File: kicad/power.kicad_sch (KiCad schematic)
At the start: 44 parts, among them J12 PJ-002B, U23 AP62300Z6, U24 AP62300Z6, U25 AP62300Z6

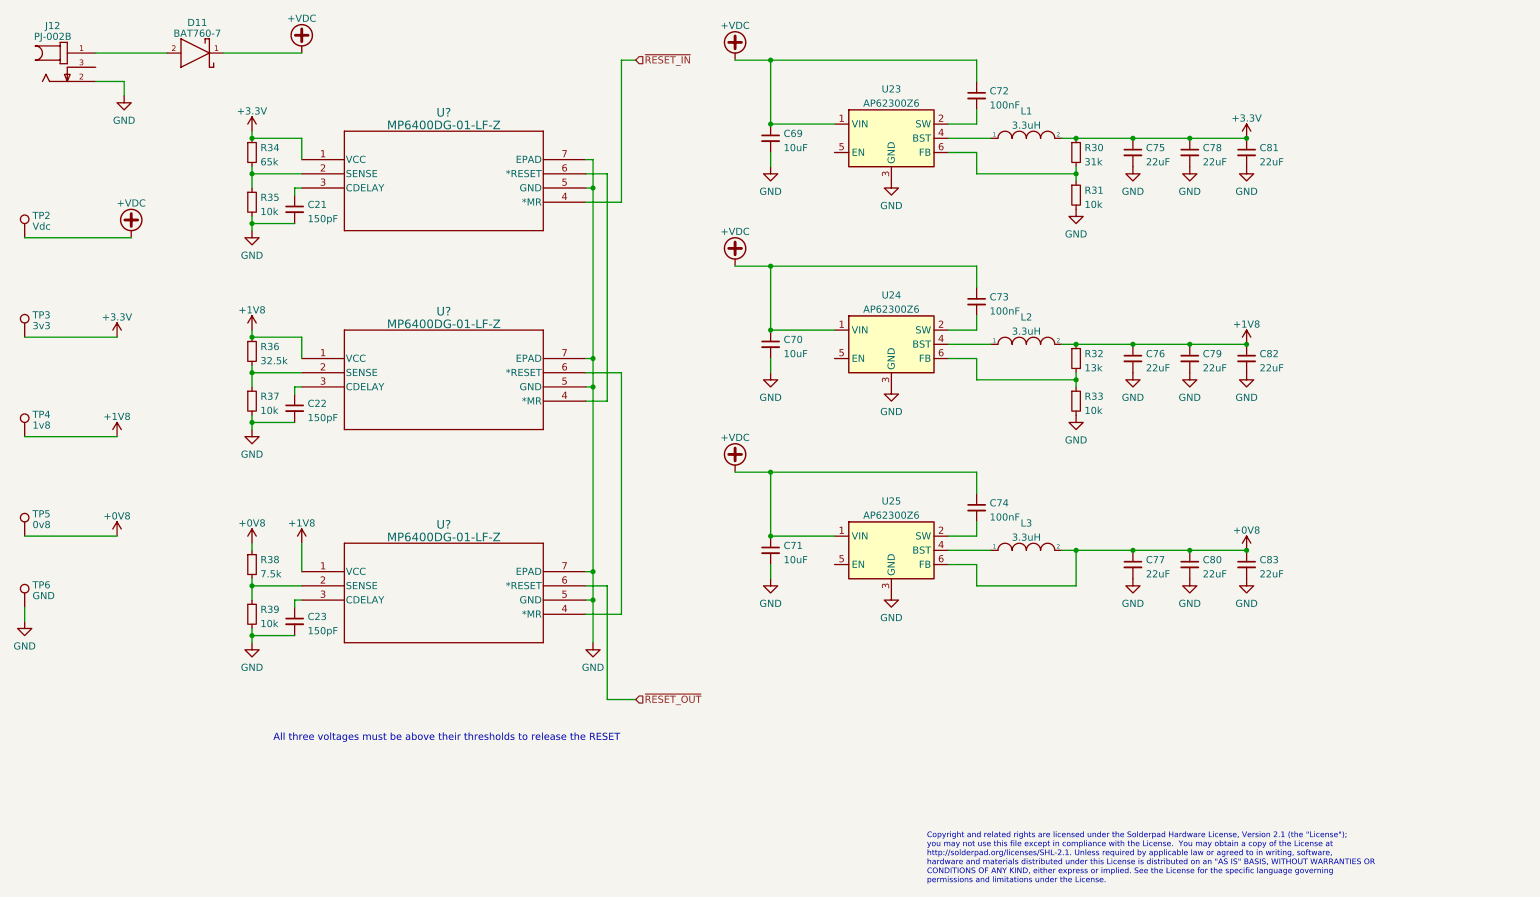
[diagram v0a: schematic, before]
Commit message: Corections made after testing V1
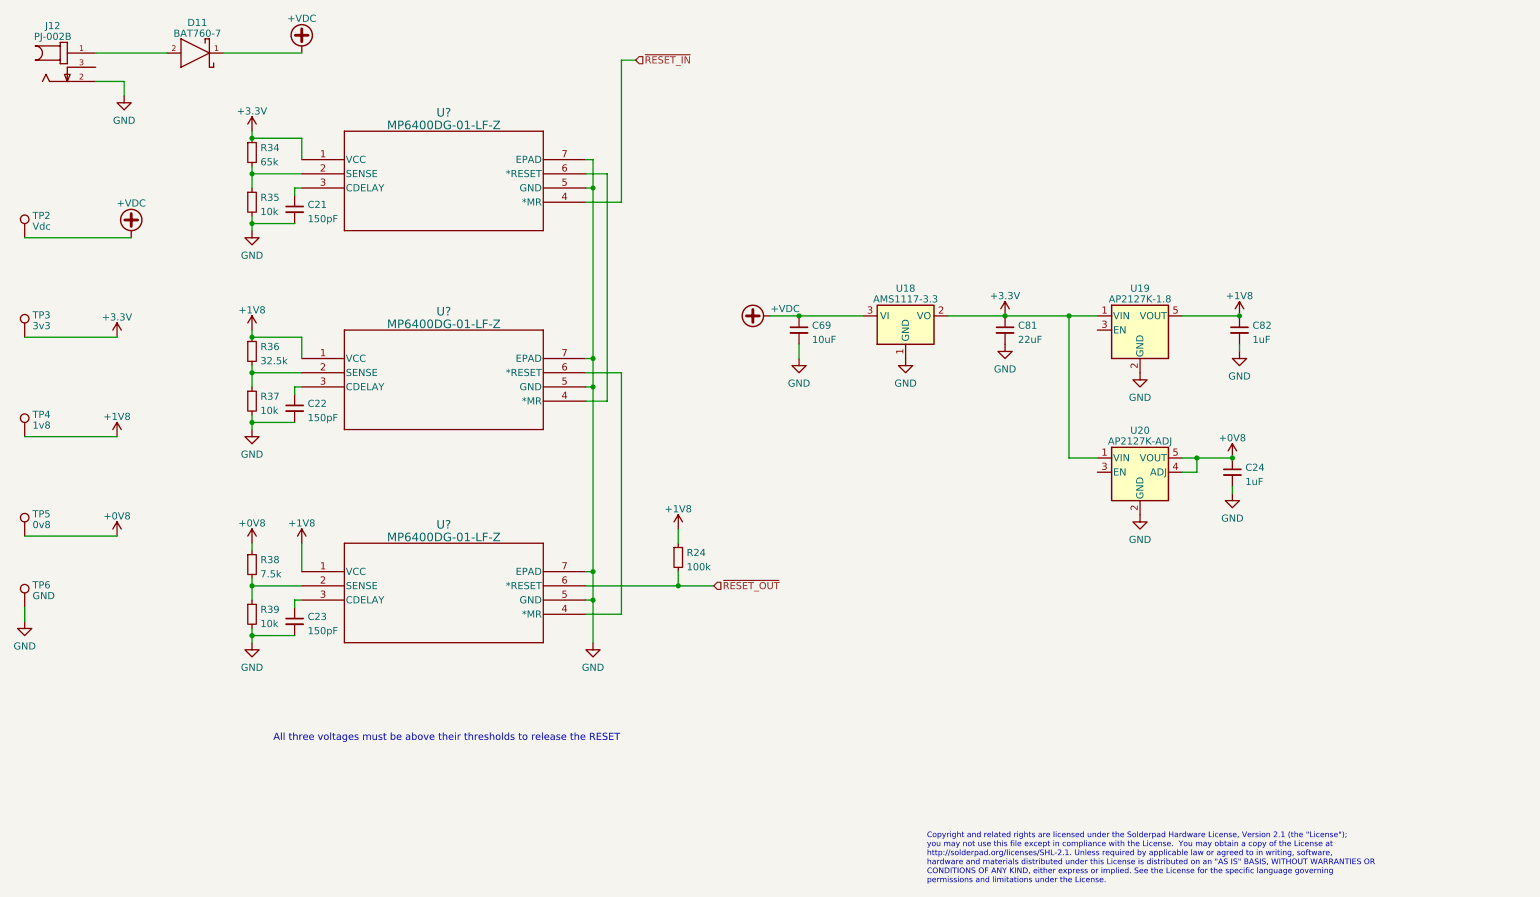
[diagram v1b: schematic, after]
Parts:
- removed C70, C71: 10uF, Capacitor_SMD:C_0603_1608Metric, symbol Device:C_Small
- removed C72, C73, C74: 100nF, Capacitor_SMD:C_0603_1608Metric, symbol Device:C_Small
- removed C75, C76, C77, C78, C79, C80, C83: 22uF, Capacitor_SMD:C_0603_1608Metric, symbol Device:C_Small
- removed L1, L2, L3: 3.3uH, Inductor_SMD:L_Bourns-SRN4018, symbol pspice:INDUCTOR
- removed R30: 31k, Resistor_SMD:R_0603_1608Metric, symbol Device:R_Small
- removed R31, R33: 10k, Resistor_SMD:R_0603_1608Metric, symbol Device:R_Small
- removed R32: 13k, Resistor_SMD:R_0603_1608Metric, symbol Device:R_Small
- removed U23, U24, U25: AP62300Z6, Package_TO_SOT_SMD:SOT-563, symbol Regulator_Switching:AP62300Z6
- added C24: 1uF, Capacitor_SMD:C_0603_1608Metric, symbol Device:C_Small
- added R24: 100k, Resistor_SMD:R_0603_1608Metric, symbol Device:R_Small
- added U18: AMS1117-3.3, Package_TO_SOT_SMD:SOT-223-3_TabPin2, symbol Regulator_Linear:AMS1117-3.3
- added U19: AP2127K-1.8, Package_TO_SOT_SMD:SOT-23-5, symbol Regulator_Linear:AP2127K-1.8
- added U20: AP2127K-ADJ, Package_TO_SOT_SMD:SOT-23-5, symbol Regulator_Linear:AP2127K-ADJ
- C82: value 22uF -> 1uF
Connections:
- net +0V8: now also C24.1, U20.4 (ADJ), U20.5 (VOUT)
- net +1V8: now also R24.1, U19.5 (VOUT)
- net +3V3: now also U18.2 (VO), U19.1 (VIN), U20.1 (VIN)
- net +VDC: now also U18.3 (VI)
- net GND: now also C24.2, U18.1 (GND), U19.2 (GND), U20.2 (GND)
- net ~{RESET_OUT}: now also R24.2
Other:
- moved on the sheet: C69, C81, C82
